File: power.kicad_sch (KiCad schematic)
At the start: 113 parts, among them J3 Conn_01x01, J4 Conn_01x01, U16 CSD95472Q5MC, U3 TPS53647, U36 MCP1824T-1202E, U4 CSD95472Q5MC, U5 CSD95472Q5MC, U6 AP3211, U7 MCP1824T-0802E

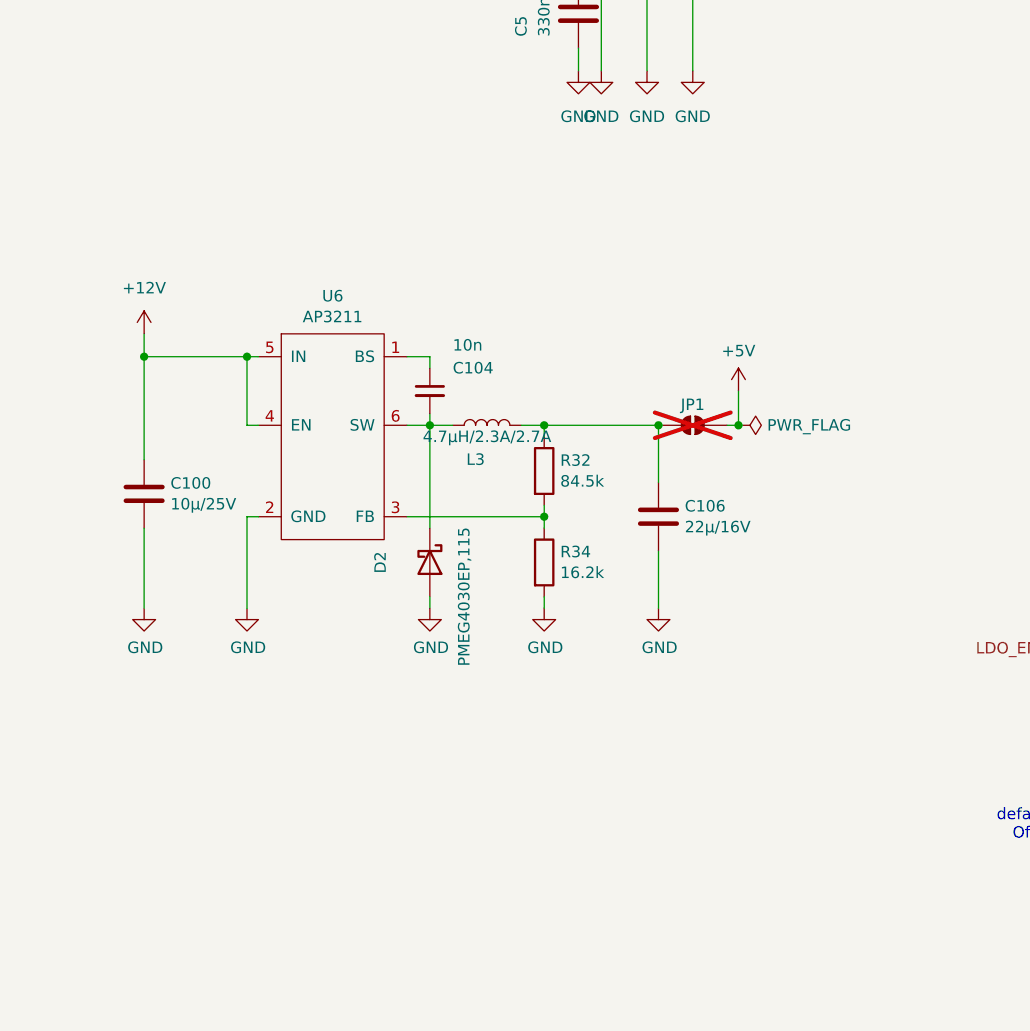
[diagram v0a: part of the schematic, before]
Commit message: sch_ should be ready
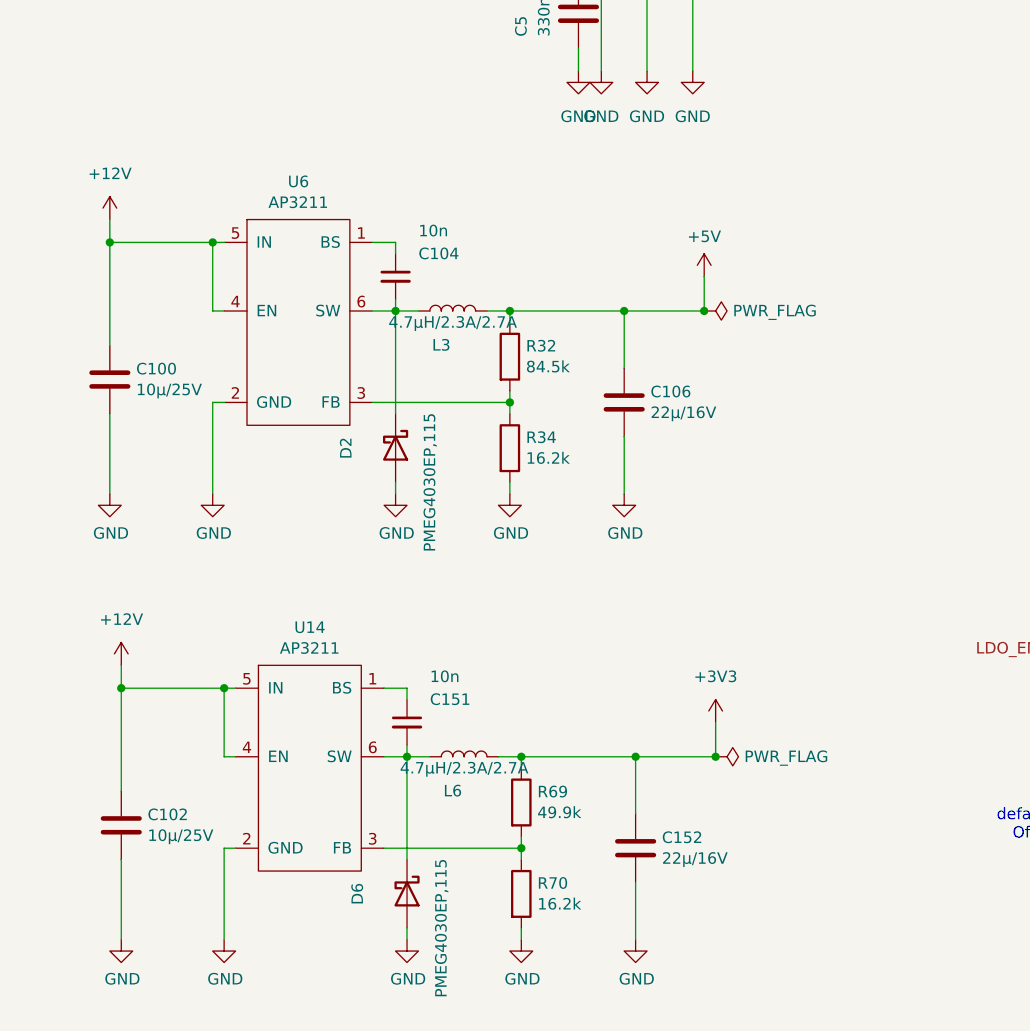
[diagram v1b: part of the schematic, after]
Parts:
- removed JP1: SolderJumper_2_Open, Jumper:SolderJumper-2_P1.3mm_Open_RoundedPad1.0x1.5mm, symbol Jumper:SolderJumper_2_Open
- added C102: 10µ/25V, Capacitor_SMD:C_0805_2012Metric, symbol Device:C
- added C151: 10n, Capacitor_SMD:C_0805_2012Metric, symbol Device:C_Small
- added C152: 22µ/16V, Capacitor_SMD:C_1206_3216Metric, symbol Device:C
- added D6: PMEG4030EP,115, Diode_SMD:D_SOD-128, symbol Device:D_Schottky
- added L6: 4.7µH/2.3A/2.7A, Inductor_SMD:L_Taiyo-Yuden_NR-50xx, symbol Device:L
- added R69: 49.9k, Resistor_SMD:R_0603_1608Metric, symbol Device:R
- added R70: 16.2k, Resistor_SMD:R_0603_1608Metric, symbol Device:R
- added U14: AP3211, Package_TO_SOT_SMD:SOT-23-6, symbol pferdibank-rescue:AP3211-mylib
- R32, R34: footprint Resistor_SMD:R_0805_2012Metric -> Resistor_SMD:R_0603_1608Metric
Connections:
- net +12V: now also C102.1, U14.4 (EN), U14.5 (IN)
- net +3V3: now also C152.1, L6.2, R69.1
- net +5V: now also C106.1, L3.2, R32.1
- net GND: now also C102.2, C152.2, D6.2 (A), R70.2, U14.2 (GND)
- new net: C151.1, U14.1 (BS)
- new net: R69.2, R70.1, U14.3 (FB)
- new net: C151.2, D6.1 (K), L6.1, U14.6 (SW)
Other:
- moved on the sheet: C100, C104, C106, D2, L3, R32, R34, U6
